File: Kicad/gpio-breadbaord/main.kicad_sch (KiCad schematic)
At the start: 10 parts, among them K1 GPIO IN, K2 GPIO OUT #3, K3 GPIO OUT #1, K4 GPIO OUT #4, K5 GPIO OUT #2

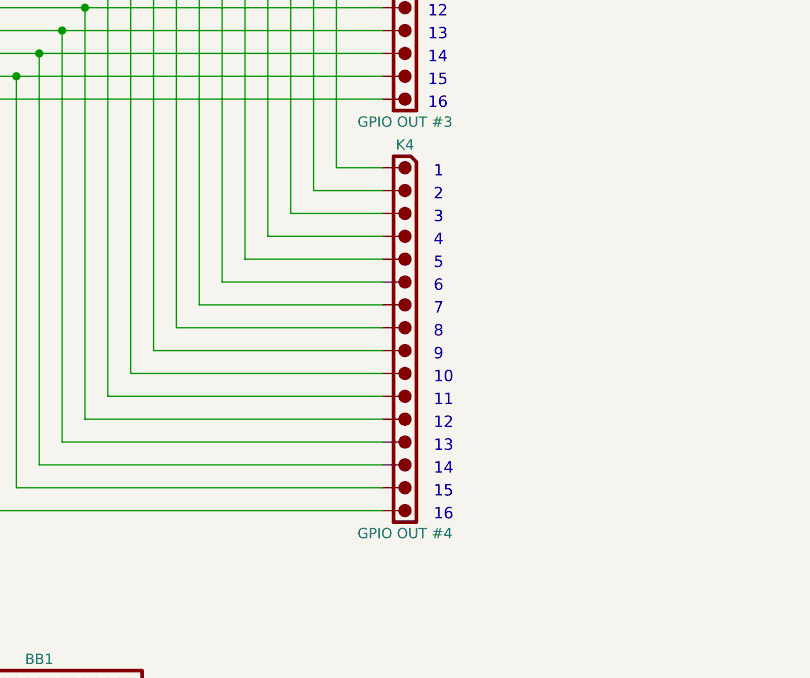
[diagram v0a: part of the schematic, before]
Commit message: Up
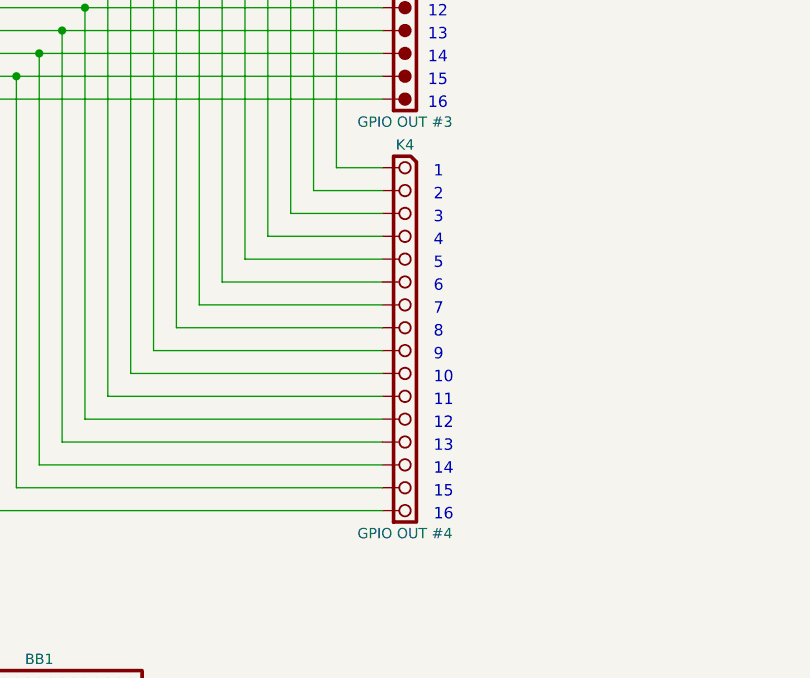
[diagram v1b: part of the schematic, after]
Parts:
- K4: footprint tronixio:HARWIN-M20-999164x -> tronixio:HARWIN-M20-782164x; symbol tronixio:HARWIN-254-M-1X16-VERTICAL -> tronixio:HARWIN-254-F-1X16-VERTICAL; Mouser 855-M20-999164 -> 855-M20-782164
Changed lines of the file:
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@@
 	)
 	(symbol
-		(lib_id "tronixio:HARWIN-254-M-1X16-VERTICAL")
+		(lib_id "tronixio:HARWIN-254-F-1X16-VERTICAL")
 		(at 190.5 78.74 0)
 		(unit 1)
@@
 			)
 		)
-		(property "Footprint" "tronixio:HARWIN-M20-999164x"
-			(at 190.5 124.46 0)
+		(property "Footprint" "tronixio:HARWIN-M20-782164x"
+			(at 190.5 121.92 0)
+			(do_not_autoplace yes)
 			(effects
 				(font
@@
 			)
 		)
-		(property "Datasheet" "https://www.harwin.com/products/M20-9991646/"
-			(at 190.5 127 0)
+		(property "Datasheet" "https://www.harwin.com/products/M20-7821646/"
+			(at 190.5 124.46 0)
+			(do_not_autoplace yes)
 			(effects
 				(font
@@
 			)
 		)
-		(property "Mouser" "855-M20-999164"
-			(at 190.5 129.54 0)
+		(property "Mouser" "855-M20-782164"
+			(at 190.5 127 0)
+			(do_not_autoplace yes)
 			(effects
 				(font
